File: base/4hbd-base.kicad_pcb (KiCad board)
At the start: 2 copper layers, 229 parts, among them J1 Spring_Terminal_Connector_01x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, J10 Spring_Terminal_Connector_01x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, J11 Spring_Terminal_Connector_01x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, J12 Spring_Terminal_Connector_01x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, J13 Screw_Terminal_01x02, J14 Conn_02x25_Odd_Even, J15 Conn_02x25_Odd_Even, J2 Spring_Terminal_Connector_01x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, J3 Spring_Terminal_Connector_01x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, J4 Spring_Terminal_Connector_01x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, J5 Spring_Terminal_Connector_01x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, J6 Spring_Terminal_Connector_01x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, J7 Screw_Terminal_01x03, J8 Spring_Terminal_Connector_01x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, J9 Spring_Terminal_Connector_01x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, Q1 irf540n, Q10 2N7002, Q11 2N7002, Q12 IRLML2060TRPBF, Q2 irf540n, Q3 irf540n, Q4 irf540n, Q5 irf540n, Q6 irf540n, Q7 irf540n, Q8 irf540n, Q9 2N7002, U1 SI8640, U10 ADS7886, U11 MOCD217M, U12 MOCD217M, U13 MOCD217M, U14 AMS1117-5.0, U15 AMS1117-5.0, U16 LM2596S-ADJ, U17 AM26LV32, U18 LM2596S-ADJ, U19 AMS1117-5.0, U2 SI8640, U20 SN65HVD230, U21 MAX485CSA, U3 IR2181, U4 IR2181, U5 IR2181, U6 IR2181, U7 ACS712xLCTR-30A, U8 ACS712xLCTR-30A, U9 ADS7886

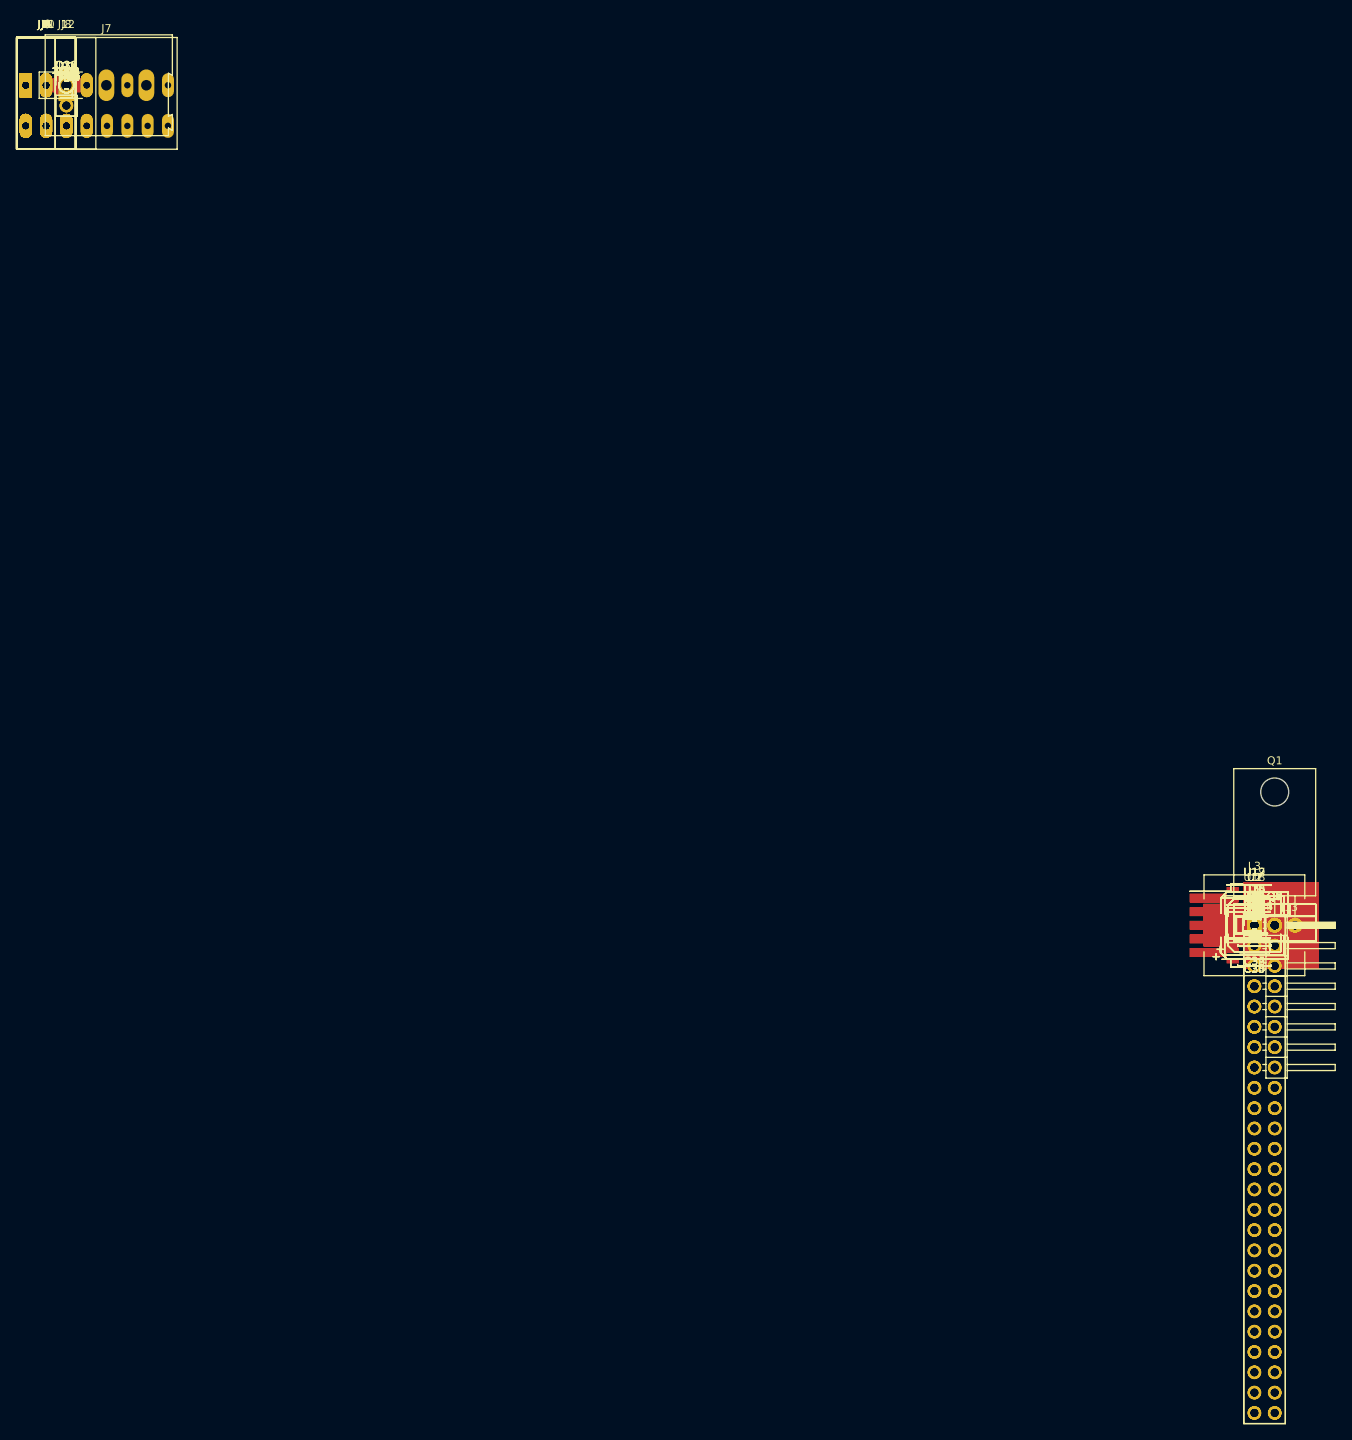
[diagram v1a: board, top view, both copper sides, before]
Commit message: fix for pcb
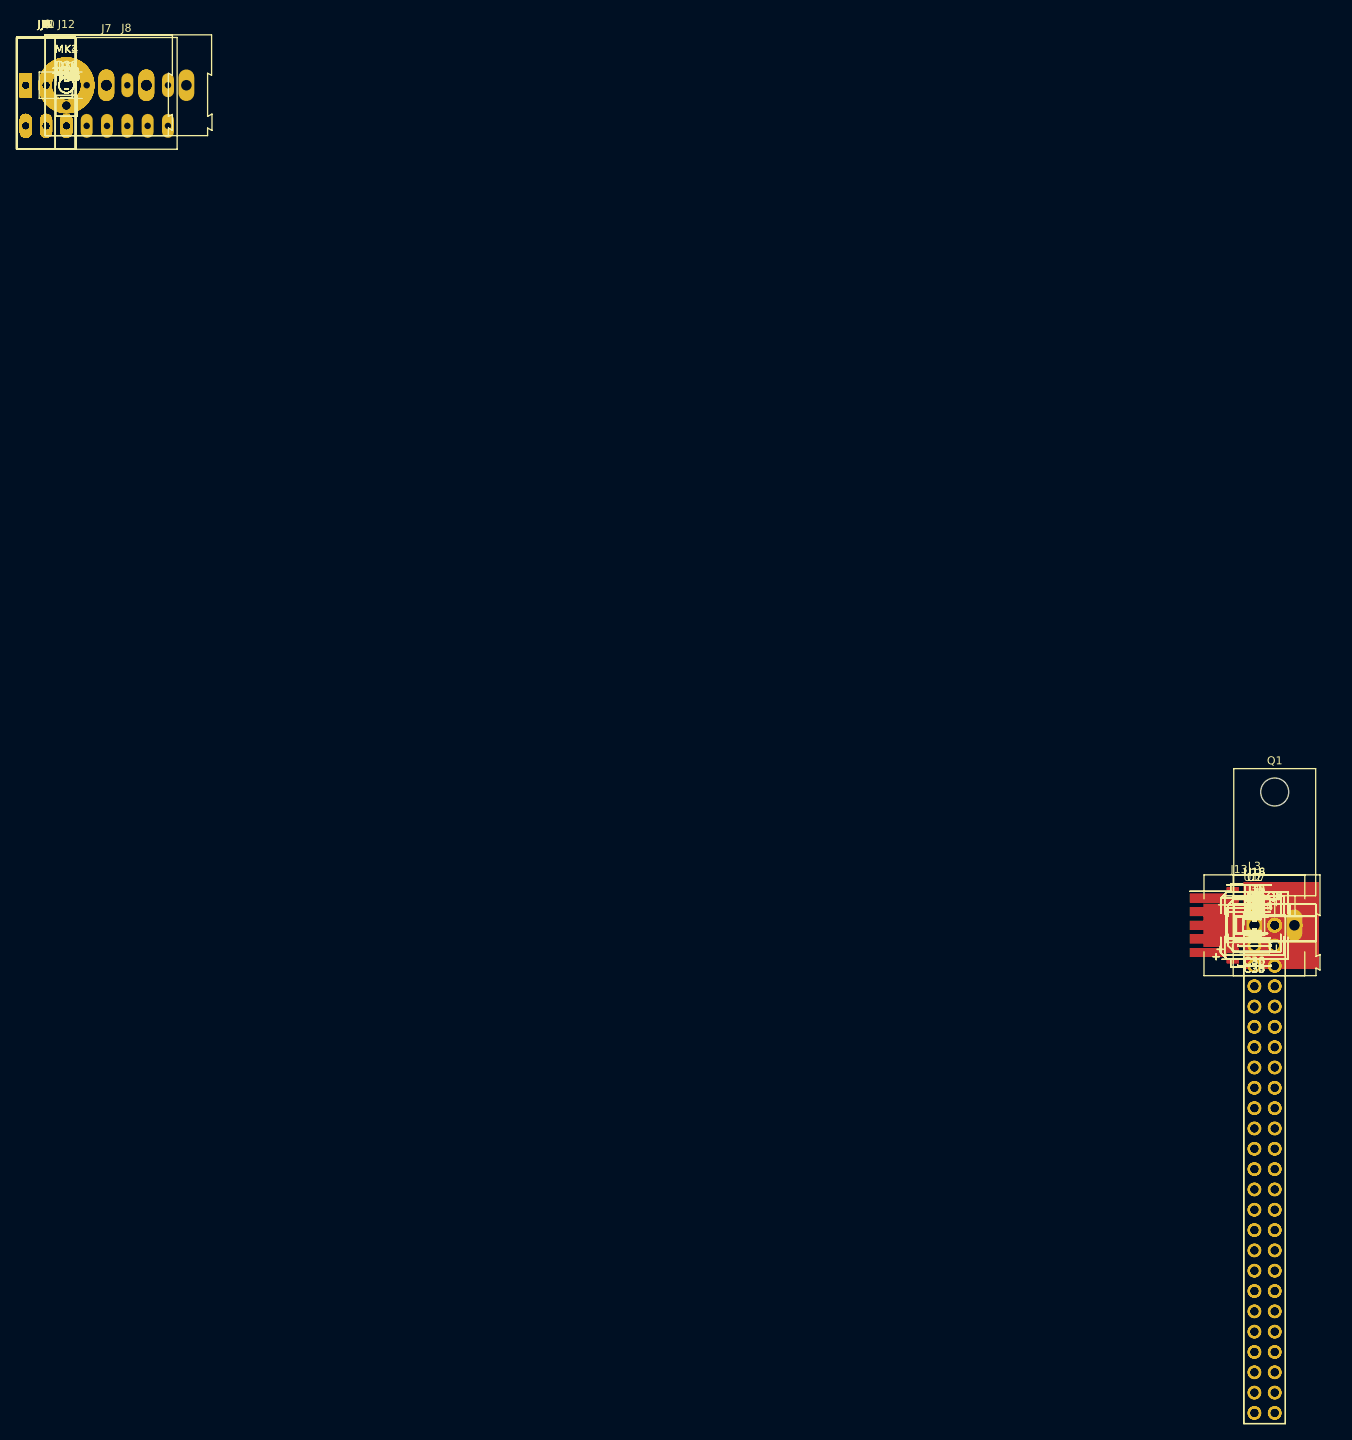
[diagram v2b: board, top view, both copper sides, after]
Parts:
- added MK1, MK2, MK3, MK4: Mounting_Hole, MountingHole:MountingHole_3.5mm_Pad, F.Cu at (0.00, 0.00)
- C19, C20, C21: footprint Capacitor_Tantalum_SMD:CP_EIA-3216-18_Kemet-A -> Capacitor_SMD:C_0805_2012Metric
- C22, C27: footprint Capacitor_SMD:C_0603_1608Metric -> Capacitor_Tantalum_SMD:CP_EIA-3216-18_Kemet-A
- C23: footprint Capacitor_SMD:CP_Elec_8x10 -> Capacitor_Tantalum_SMD:CP_EIA-3216-18_Kemet-A
- C24: footprint Capacitor_Tantalum_SMD:CP_EIA-3216-18_Kemet-A -> Capacitor_SMD:C_0603_1608Metric
- C25: footprint Capacitor_Tantalum_SMD:CP_EIA-3216-18_Kemet-A -> Capacitor_SMD:CP_Elec_8x10
- C37: footprint Capacitor_SMD:CP_Elec_6.3x7.7 -> Capacitor_SMD:C_0603_1608Metric
- C38: footprint Capacitor_SMD:CP_Elec_6.3x5.3 -> Capacitor_SMD:CP_Elec_6.3x7.7
- C40: footprint Capacitor_SMD:C_0603_1608Metric -> Capacitor_SMD:CP_Elec_6.3x5.3
- D21: footprint Diode_SMD:D_SMA -> Diode_SMD:D_SOD-123
- D22, D27: footprint Diode_SMD:D_SMB -> Diode_SMD:D_SOD-123
- D23: footprint Diode_SMD:D_SOD-123 -> Diode_SMD:D_SMA
- D24: footprint Diode_SMD:D_SMA -> Diode_SMD:D_SMB
- D29: footprint Package_TO_SOT_SMD:SOT-23 -> Diode_SMD:D_SMB
- J13: footprint Connector_PinHeader_2.54mm:PinHeader_1x08_P2.54mm_Horizontal -> TerminalBlock:TerminalBlock_Altech_AK300-2_P5.00mm
- J8: value Spring_Terminal_Connector_01x04 -> Screw_Terminal_01x04; footprint TerminalBlock:SpringTerminalBlock_KF141R_4_P2.54mm -> TerminalBlock:TerminalBlock_Altech_AK300-4_P5.00mm
- R35, R36: footprint Resistor_SMD:R_0603_1608Metric -> Resistor_SMD:R_0805_2012Metric
- U16: footprint Package_TO_SOT_SMD:SOT-223 -> Package_TO_SOT_SMD:TO-263-5_TabPin3
- U17: footprint Package_TO_SOT_SMD:TO-263-5_TabPin3 -> Package_SOIC:SOIC-16_3.9x9.9mm_P1.27mm
- U18: footprint Package_SOIC:SOIC-16_3.9x9.9mm_P1.27mm -> Package_TO_SOT_SMD:TO-263-5_TabPin3
- U19: footprint Package_TO_SOT_SMD:TO-263-5_TabPin3 -> Package_TO_SOT_SMD:SOT-223
- U20: footprint Package_TO_SOT_SMD:SOT-223 -> Package_SOIC:SOIC-8_3.9x4.9mm_P1.27mm
- U21: footprint Package_SOIC:SOIC-8_3.9x4.9mm_P1.27mm -> Package_SOIC:SO-8_5.3x6.2mm_P1.27mm
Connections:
- J14 pad 1: Net-(J14-Pad1) -> (no net)
- J14 pad 12: Net-(J14-Pad12) -> (no net)
- J14 pad 13: Net-(J14-Pad13) -> (no net)
- J14 pad 14: Net-(J14-Pad14) -> (no net)
- J14 pad 16: Net-(J14-Pad16) -> (no net)
- J14 pad 18: Net-(J14-Pad18) -> (no net)
- J14 pad 2: Net-(J14-Pad2) -> (no net)
- J14 pad 20: Net-(J14-Pad20) -> (no net)
- J14 pad 21: Net-(J14-Pad21) -> (no net)
- J14 pad 26: Net-(J14-Pad26) -> (no net)
- J14 pad 3: Net-(J14-Pad3) -> (no net)
- J14 pad 32: Net-(J14-Pad32) -> (no net)
- J14 pad 35: Net-(J14-Pad35) -> (no net)
- J14 pad 37: Net-(J14-Pad37) -> (no net)
- J14 pad 4: Net-(J14-Pad4) -> (no net)
- J14 pad 46: /MCU/FPGA connection/PWM_Trip -> (no net)
- J14 pad 47: Net-(J14-Pad47) -> (no net)
- J14 pad 48: Net-(J14-Pad48) -> (no net)
- J14 pad 5: Net-(J14-Pad5) -> (no net)
- J14 pad 6: Net-(J14-Pad6) -> (no net)
- J14 pad 7: Net-(J14-Pad7) -> (no net)
- J14 pad 8: Net-(J14-Pad8) -> (no net)
- J14 pad 9: Net-(J14-Pad9) -> (no net)
- J15 pad 10: Net-(J15-Pad10) -> (no net)
- J15 pad 11: Net-(J15-Pad11) -> (no net)
- J15 pad 12: Net-(J15-Pad12) -> (no net)
- J15 pad 14: Net-(J15-Pad14) -> (no net)
- J15 pad 15: Net-(J15-Pad15) -> (no net)
- J15 pad 16: Net-(J15-Pad16) -> (no net)
- J15 pad 17: Net-(J15-Pad17) -> (no net)
- J15 pad 18: Net-(J15-Pad18) -> (no net)
- J15 pad 19: Net-(J15-Pad19) -> (no net)
- J15 pad 20: Net-(J15-Pad20) -> (no net)
- J15 pad 21: Net-(J15-Pad21) -> (no net)
- J15 pad 22: Net-(J15-Pad22) -> (no net)
- J15 pad 26: Net-(J15-Pad26) -> (no net)
- J15 pad 27: Net-(J15-Pad27) -> (no net)
- J15 pad 28: Net-(J15-Pad28) -> (no net)
- J15 pad 29: Net-(J15-Pad29) -> (no net)
- J15 pad 30: Net-(J15-Pad30) -> (no net)
- J15 pad 37: Net-(J15-Pad37) -> (no net)
- J15 pad 38: Net-(J15-Pad38) -> (no net)
- J15 pad 39: Net-(J15-Pad39) -> (no net)
- J15 pad 4: Net-(J15-Pad4) -> (no net)
- J15 pad 40: Net-(J15-Pad40) -> (no net)
- J15 pad 44: Net-(J15-Pad44) -> (no net)
- J15 pad 47: Net-(J15-Pad47) -> (no net)
- J15 pad 48: Net-(J15-Pad48) -> (no net)
- J15 pad 5: Net-(J15-Pad5) -> (no net)
- J15 pad 6: Net-(J15-Pad6) -> (no net)
- J15 pad 7: Net-(J15-Pad7) -> (no net)
- J15 pad 8: Net-(J15-Pad8) -> (no net)
- Q9 pad 1: Net-(Q9-Pad1) -> (no net)
- Q9 pad 2: Net-(Q9-Pad2) -> (no net)
- Q9 pad 3: Net-(Q9-Pad3) -> (no net)
